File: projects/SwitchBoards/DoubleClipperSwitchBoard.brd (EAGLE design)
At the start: 18.2 x 16.9 mm, 12 parts

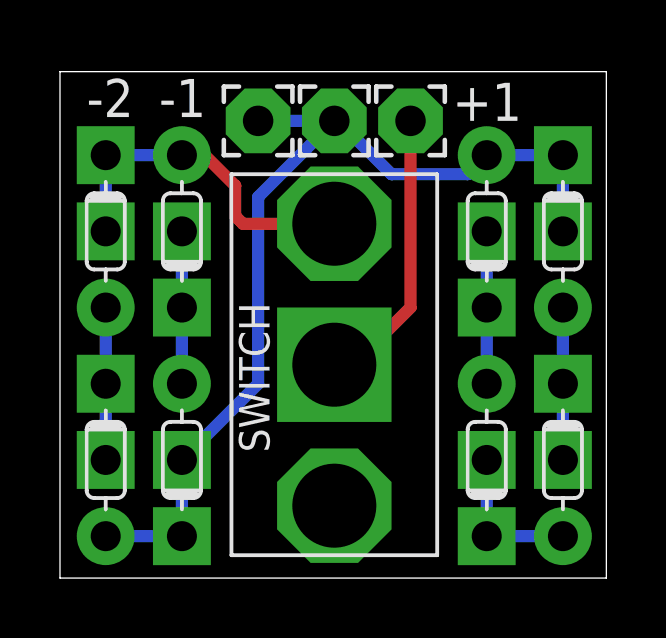
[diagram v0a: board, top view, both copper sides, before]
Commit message: Final project updates. Ready to send to oshpark.
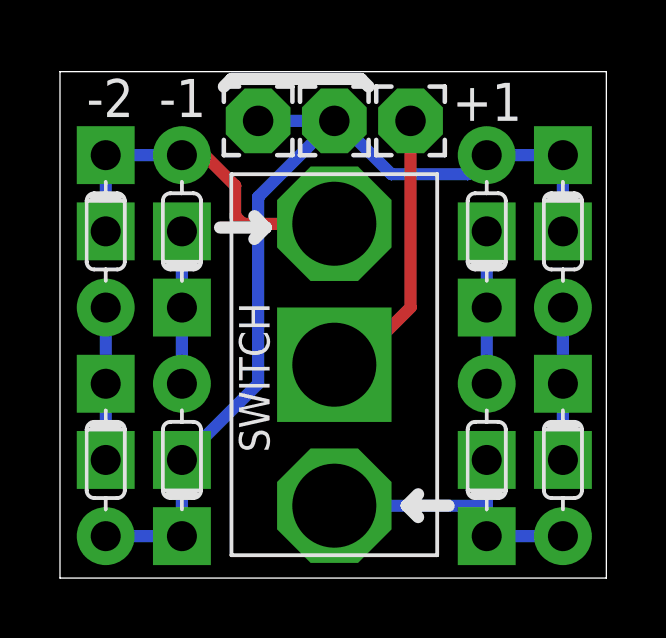
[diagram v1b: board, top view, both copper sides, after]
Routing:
- net N$3: track 5.08 -> 10.2 mm
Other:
- board text added: "GJCAMANN(C)2014"
- board text added: "V1.0"
- board text removed: "GJCAMANN1/2014"
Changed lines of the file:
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@@
 <layer number="27" name="tValues" color="7" fill="1" visible="yes" active="yes"/>
 <layer number="28" name="bValues" color="7" fill="1" visible="yes" active="yes"/>
-<layer number="29" name="tStop" color="7" fill="3" visible="no" active="yes"/>
-<layer number="30" name="bStop" color="7" fill="6" visible="no" active="yes"/>
-<layer number="31" name="tCream" color="7" fill="4" visible="no" active="yes"/>
-<layer number="32" name="bCream" color="7" fill="5" visible="no" active="yes"/>
-<layer number="33" name="tFinish" color="6" fill="3" visible="no" active="yes"/>
-<layer number="34" name="bFinish" color="6" fill="6" visible="no" active="yes"/>
-<layer number="35" name="tGlue" color="7" fill="4" visible="no" active="yes"/>
-<layer number="36" name="bGlue" color="7" fill="5" visible="no" active="yes"/>
-<layer number="37" name="tTest" color="7" fill="1" visible="no" active="yes"/>
-<layer number="38" name="bTest" color="7" fill="1" visible="no" active="yes"/>
+<layer number="29" name="tStop" color="7" fill="3" visible="yes" active="yes"/>
+<layer number="30" name="bStop" color="7" fill="6" visible="yes" active="yes"/>
+<layer number="31" name="tCream" color="7" fill="4" visible="yes" active="yes"/>
+<layer number="32" name="bCream" color="7" fill="5" visible="yes" active="yes"/>
+<layer number="33" name="tFinish" color="6" fill="3" visible="yes" active="yes"/>
+<layer number="34" name="bFinish" color="6" fill="6" visible="yes" active="yes"/>
+<layer number="35" name="tGlue" color="7" fill="4" visible="yes" active="yes"/>
+<layer number="36" name="bGlue" color="7" fill="5" visible="yes" active="yes"/>
+<layer number="37" name="tTest" color="7" fill="1" visible="yes" active="yes"/>
+<layer number="38" name="bTest" color="7" fill="1" visible="yes" active="yes"/>
 <layer number="39" name="tKeepout" color="4" fill="11" visible="yes" active="yes"/>
 <layer number="40" name="bKeepout" color="1" fill="11" visible="yes" active="yes"/>
@@
 <layer number="42" name="bRestrict" color="1" fill="10" visible="yes" active="yes"/>
 <layer number="43" name="vRestrict" color="2" fill="10" visible="yes" active="yes"/>
-<layer number="44" name="Drills" color="7" fill="1" visible="no" active="yes"/>
-<layer number="45" name="Holes" color="7" fill="1" visible="no" active="yes"/>
-<layer number="46" name="Milling" color="3" fill="1" visible="no" active="yes"/>
-<layer number="47" name="Measures" color="7" fill="1" visible="no" active="yes"/>
+<layer number="44" name="Drills" color="7" fill="1" visible="yes" active="yes"/>
+<layer number="45" name="Holes" color="7" fill="1" visible="yes" active="yes"/>
+<layer number="46" name="Milling" color="3" fill="1" visible="yes" active="yes"/>
+<layer number="47" name="Measures" color="7" fill="1" visible="yes" active="yes"/>
 <layer number="48" name="Document" color="7" fill="1" visible="yes" active="yes"/>
 <layer number="49" name="Reference" color="7" fill="1" visible="yes" active="yes"/>
@@
 <wire x1="18.212" y1="16.881" x2="0" y2="16.881" width="0" layer="20"/>
 <wire x1="0" y1="16.881" x2="0" y2="0" width="0" layer="20"/>
-<text x="11.43" y="0.889" size="1.016" layer="22" rot="MR90">GJCAMANN1/2014</text>
+<text x="11.43" y="0.889" size="1.016" layer="22" rot="MR90">GJCAMANN(C)2014</text>
 <text x="5.842" y="0.254" size="1.016" layer="22" rot="MR90">DoubleClipperSwitch</text>
+<text x="17.78" y="15.24" size="1.016" layer="22" rot="MR0">V1.0</text>
+<wire x1="5.334" y1="11.684" x2="6.858" y2="11.684" width="0.4064" layer="21"/>
+<wire x1="6.477" y1="12.065" x2="6.858" y2="11.684" width="0.4064" layer="21"/>
+<wire x1="6.858" y1="11.684" x2="6.477" y2="11.303" width="0.4064" layer="21"/>
+<wire x1="12.954" y1="2.413" x2="11.557" y2="2.413" width="0.4064" layer="21"/>
+<wire x1="11.938" y1="2.794" x2="11.557" y2="2.413" width="0.4064" layer="21"/>
+<wire x1="11.938" y1="2.032" x2="11.557" y2="2.413" width="0.4064" layer="21"/>
+<wire x1="10.287" y1="16.383" x2="10.033" y2="16.637" width="0.4064" layer="21"/>
+<wire x1="10.033" y1="16.637" x2="5.715" y2="16.637" width="0.4064" layer="21"/>
+<wire x1="5.715" y1="16.637" x2="5.461" y2="16.383" width="0.4064" layer="21"/>
 </plain>
 <attributes>
@@
 <contactref element="U$1" pad="P$1"/>
 <wire x1="14.224" y1="1.397" x2="16.764" y2="1.397" width="0.4064" layer="16"/>
-<wire x1="14.224" y1="1.397" x2="14.224" y2="3.937" width="0.4064" layer="16"/>
-<wire x1="9.144" y1="2.413" x2="14.224" y2="3.937" width="0" layer="19" extent="1-1"/>
+<wire x1="14.224" y1="1.397" x2="14.224" y2="2.413" width="0.4064" layer="16"/>
+<wire x1="14.224" y1="2.54" x2="14.224" y2="3.937" width="0.4064" layer="16"/>
+<wire x1="9.144" y1="2.413" x2="14.224" y2="2.413" width="0.4064" layer="16"/>
+<wire x1="14.224" y1="2.413" x2="14.224" y2="2.54" width="0.4064" layer="16"/>
 </signal>
 <signal name="N$4">
